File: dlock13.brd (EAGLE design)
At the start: 100 x 80 mm, 17 parts, among them IC2 7805T, Q1 IRLZ44Z, Q2 IRLZ44Z

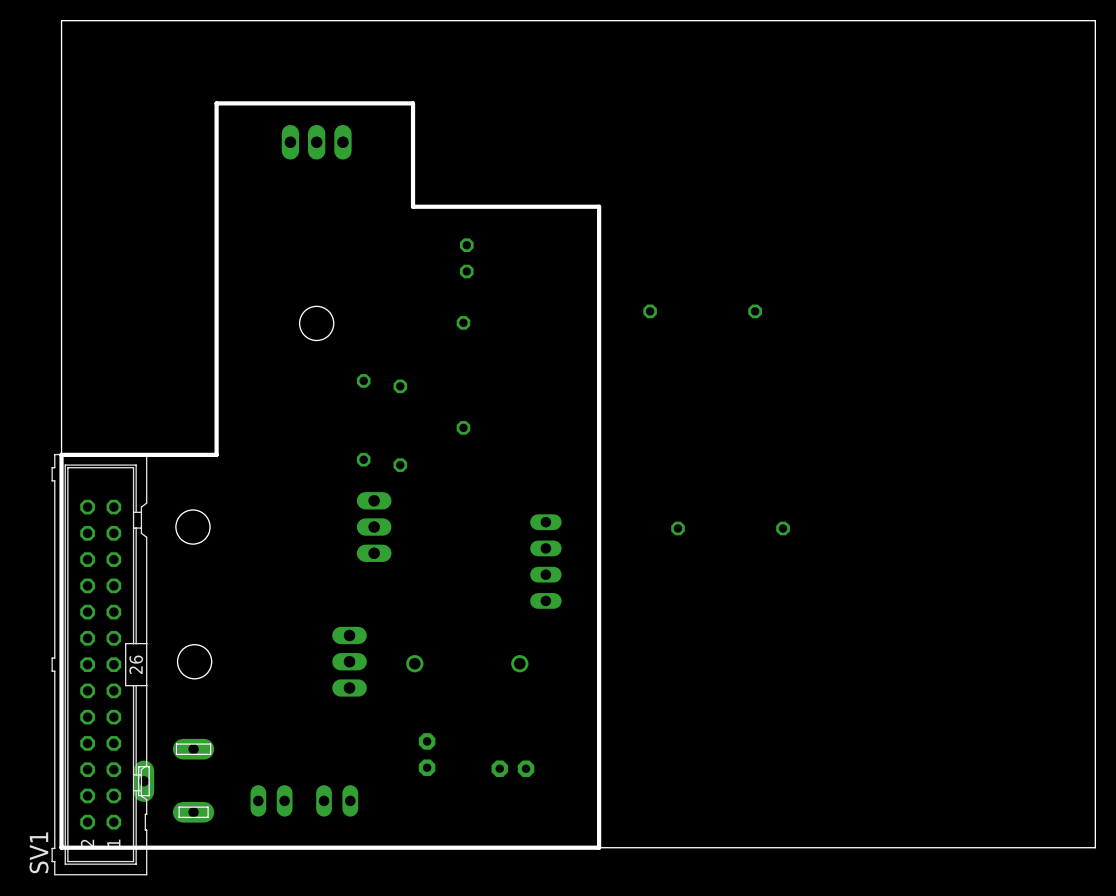
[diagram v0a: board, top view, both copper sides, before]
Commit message: Add vidarkr's changes. Produced and In use.
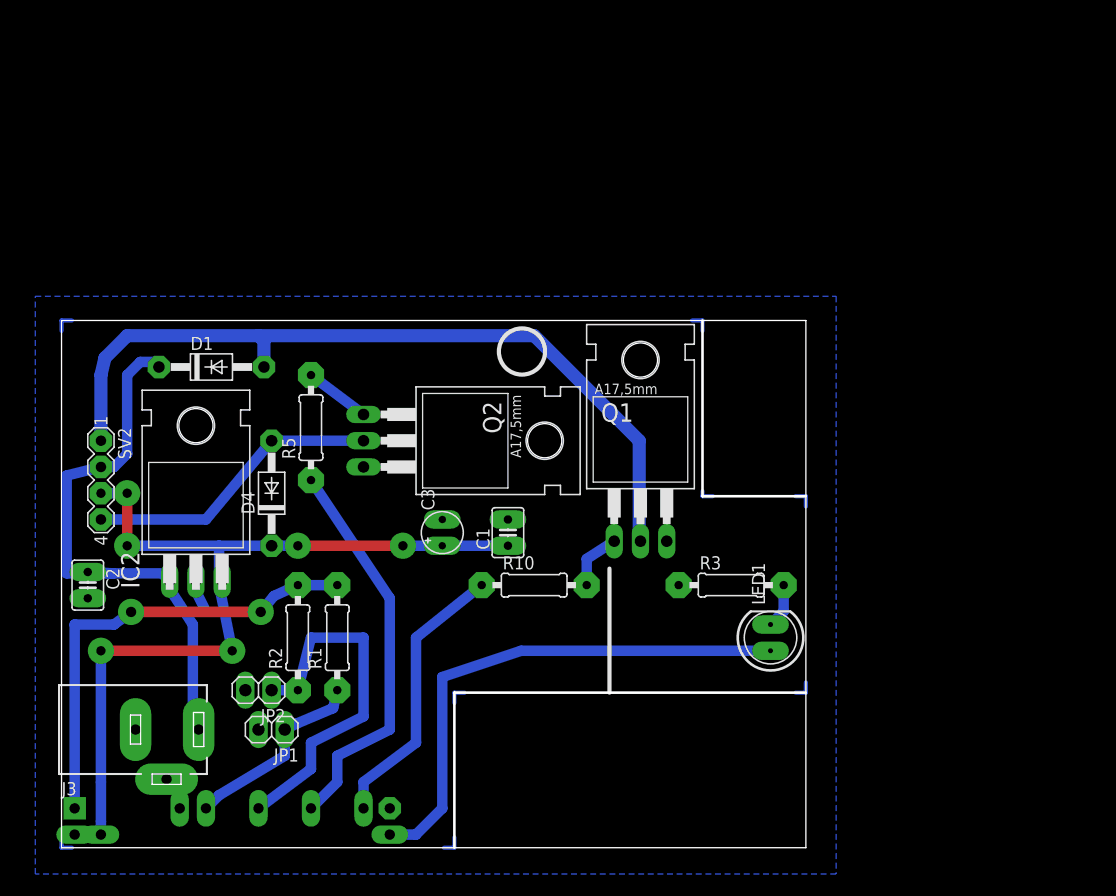
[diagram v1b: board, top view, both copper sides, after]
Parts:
- removed SV1: (no value), con-ml:ML26
- added C3: (no value), rcl:E1,8-4
- added D1: 1N4004DO41-10LARGEPADS, diode:DO41-10
- added PICONNECTOR: RASPBERRY-PI, RaspberryPi:RASPBERRY-PI_REV1
- D4: value 1N4004 -> 1N4004DO41-10LARGEPADS
- R10, R5: device resistor:0204/7 -> rcl:0207/10
- moved R2 50.3 mm to (22.9, 20.3), flipped to the top, turned to 90 degrees
- moved LED1 47.0 mm to (68.6, 20.3), flipped to the top, turned to 90 degrees
- moved SV2 43.8 mm to (3.81, 35.6), flipped to the top
- moved Q1 40.6 mm to (56.0, 36.0), flipped to the top, turned to 0 degrees
- moved R1 39.5 mm to (26.7, 20.3), flipped to the top, turned to 90 degrees
- moved C2 36.7 mm to (2.54, 25.4), flipped to the top
- moved R3 32.9 mm to (64.8, 25.4), flipped to the top, turned to 0 degrees
- moved D4 25.1 mm to (20.3, 34.3), flipped to the top, turned to 90 degrees
- moved R10 22.9 mm to (45.7, 25.4), flipped to the top, turned to 0 degrees
- moved C1 22.8 mm to (43.2, 30.5), flipped to the top, turned to 90 degrees
- moved IC2 18.6 mm to (13.0, 36.0), flipped to the top, turned to 0 degrees
- moved Q2 14.3 mm to (35.6, 39.4), flipped to the top
- moved JP2 10.8 mm to (19.1, 15.2), flipped to the top, turned to 180 degrees
- moved JP1 9.37 mm to (20.3, 11.4), flipped to the top, turned to 180 degrees
- moved R5 8.64 mm to (24.1, 40.6), flipped to the top, turned to 90 degrees
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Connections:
- removed net N$1: R5.1, SV1.22
- removed net N$12: JP2.1, SV1.15
- removed net N$8: JP1.1, R1.1, SV1.16
- removed net N$9: LED1.A, SV1.26
- new net GPI10_OUTERDOOR: PICONNECTOR.19, R5.1
- new net GPIO11_INNERDOOR: PICONNECTOR.23, R10.1
- new net GPIO17_J1: JP1.1, PICONNECTOR.11, R1.1
- new net GPIO22_J2: JP2.1, PICONNECTOR.15, R2.1
- net +12V: now also D1.C
- net +3V3: now also PICONNECTOR.1; no longer SV1.1
- net GND: now also C3.-, PICONNECTOR.25, PICONNECTOR.9; no longer SV1.25
- net N$13: now also LED1.A, PICONNECTOR.26; no longer Q1.D, SV2.1
- net N$2: now also D1.A, Q1.D, SV2.1; no longer R10.1, SV1.18
- net VCC: now also C3.+, PICONNECTOR.2, PICONNECTOR.4; no longer SV1.2
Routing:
- net VCC: track 0.00 -> 88.2 mm, vias 0 -> 6
- net N$2: track 0.00 -> 77.9 mm
- net +12V: track 0.00 -> 55.9 mm
- net N$13: track 0.00 -> 51.0 mm
- net +3V3: track 0.00 -> 44.5 mm, vias 0 -> 2
- net GPI10_OUTERDOOR: track 0.00 -> 38.2 mm
- net GPIO22_J2: track 0.00 -> 35.0 mm
- net N$14: track 0.00 -> 29.0 mm
- net GPIO11_INNERDOOR: track 0.00 -> 27.2 mm
- net GPIO17_J1: track 0.00 -> 18.6 mm
- net N$7: track 0.00 -> 6.35 mm
- net N$4: track 0.00 -> 5.70 mm
- net N$11: track 0.00 -> 4.34 mm
- net N$15: track 0.00 -> 2.84 mm
- net N$9: track 0.00 -> 2.00 mm
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- added copper zone on layer 16, net GND
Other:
- board size 100 x 80 mm -> 72 x 51 mm
